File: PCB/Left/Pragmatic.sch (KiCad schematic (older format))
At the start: 75 parts, among them J1 Conn_02x07_Odd_Even, SW1 SW_Push, SW10 SW_Push, SW11 SW_Push, SW12 SW_Push, SW13 SW_Push, SW14 SW_Push, SW15 SW_Push, SW16 SW_Push, SW17 SW_Push, SW18 SW_Push, SW19 SW_Push, SW2 SW_Push, SW20 SW_Push, SW21 SW_Push, SW22 SW_Push, SW23 SW_Push, SW24 SW_Push, SW25 SW_Push, SW26 SW_Push, SW27 SW_Push, SW28 SW_Push, SW29 SW_Push, SW3 SW_Push, SW30 SW_Push, SW31 SW_Push, SW32 SW_Push, SW33 SW_Push, SW34 SW_Push, SW35 SW_Push, SW36 SW_Push, SW4 SW_Push, SW5 SW_Push, SW6 SW_Push, SW7 SW_Push, SW8 SW_Push, SW9 SW_Push

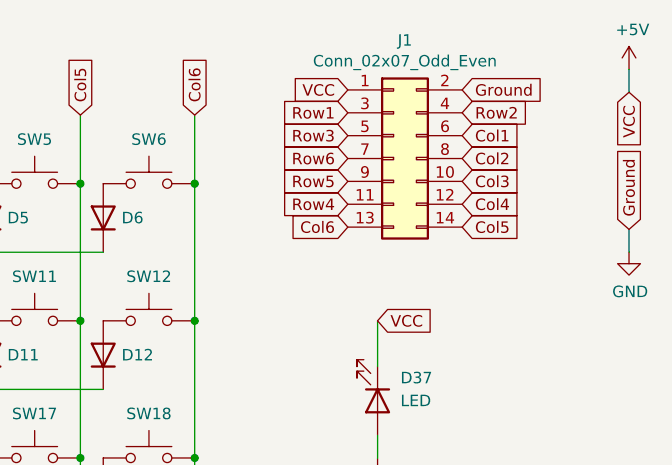
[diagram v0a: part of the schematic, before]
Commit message: left ready
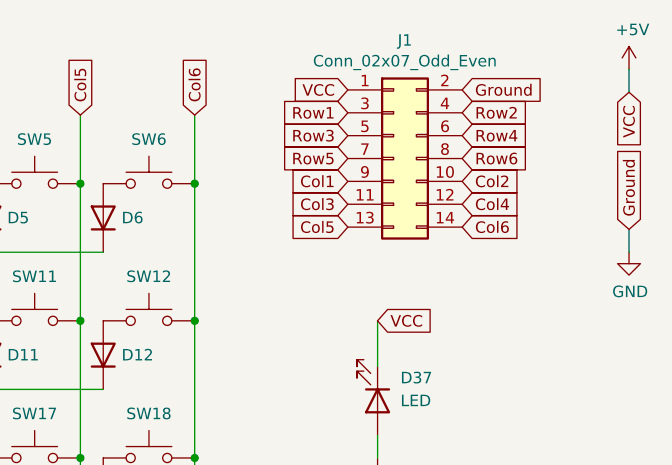
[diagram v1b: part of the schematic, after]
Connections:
- net Col1: now also J1.9 (Pin_9); no longer J1.6 (Pin_6)
- net Col2: now also J1.10 (Pin_10); no longer J1.8 (Pin_8)
- net Col3: now also J1.11 (Pin_11); no longer J1.10 (Pin_10)
- net Col5: now also J1.13 (Pin_13); no longer J1.14 (Pin_14)
- net Col6: now also J1.14 (Pin_14); no longer J1.13 (Pin_13)
- net Row4: now also J1.6 (Pin_6); no longer J1.11 (Pin_11)
- net Row5: now also J1.7 (Pin_7); no longer J1.9 (Pin_9)
- net Row6: now also J1.8 (Pin_8); no longer J1.7 (Pin_7)
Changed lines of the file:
@@
 Text GLabel 6070 2590 2    50   Input ~ 0
 Ground
-Text GLabel 6070 2790 2    50   Input ~ 0
+Text GLabel 5570 2990 0    50   Input ~ 0
 Col1
-Text GLabel 6070 2890 2    50   Input ~ 0
+Text GLabel 6070 2990 2    50   Input ~ 0
 Col2
+Text GLabel 6070 3190 2    50   Input ~ 0
+Col6
 Text GLabel 5570 3190 0    50   Input ~ 0
-Col6
-Text GLabel 6070 3190 2    50   Input ~ 0
 Col5
 Text GLabel 6070 3090 2    50   Input ~ 0
 Col4
-Text GLabel 6070 2990 2    50   Input ~ 0
+Text GLabel 5570 3090 0    50   Input ~ 0
 Col3
-Text GLabel 5570 3090 0    50   Input ~ 0
+Text GLabel 6070 2790 2    50   Input ~ 0
 Row4
-Text GLabel 5570 2990 0    50   Input ~ 0
+Text GLabel 5570 2890 0    50   Input ~ 0
 Row5
-Text GLabel 5570 2890 0    50   Input ~ 0
+Text GLabel 6070 2890 2    50   Input ~ 0
 Row6
 $Comp
